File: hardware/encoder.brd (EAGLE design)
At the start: 26.2 x 31.4 mm, 13 parts

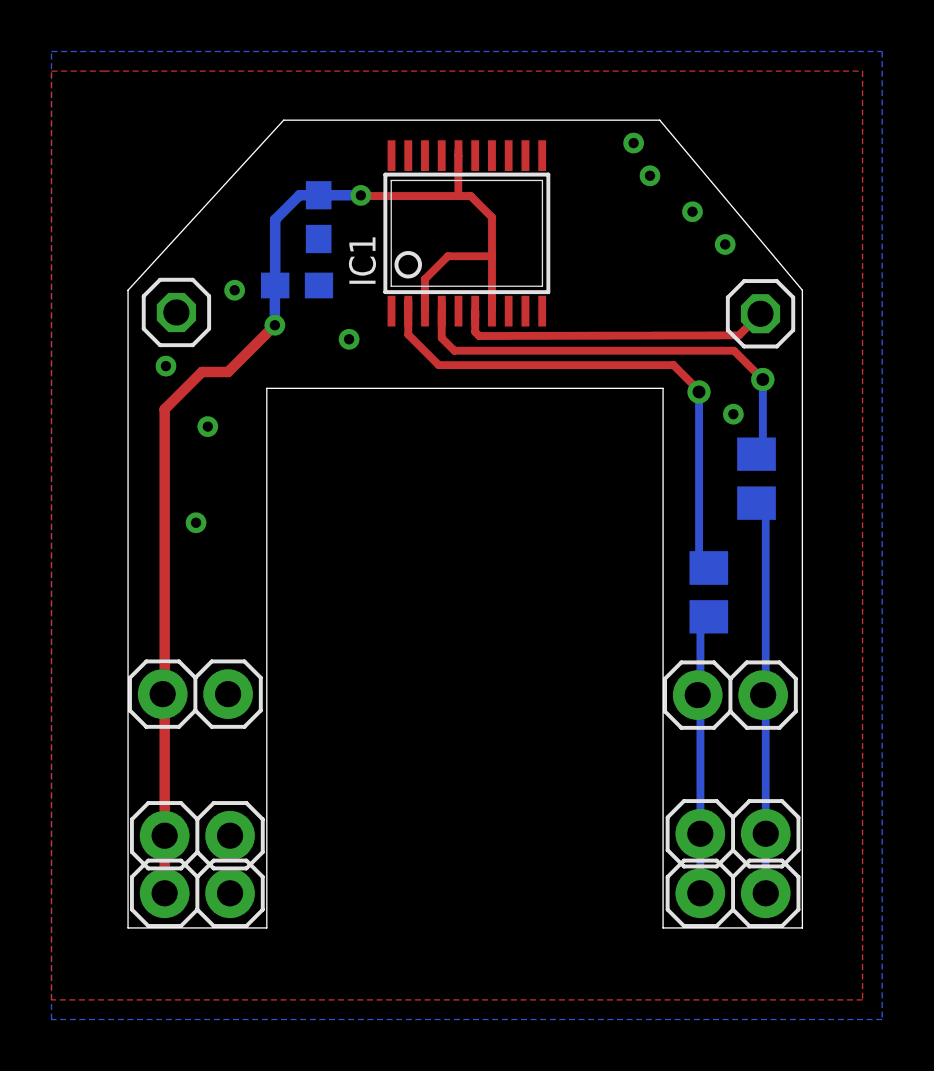
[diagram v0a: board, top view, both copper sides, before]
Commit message: new driver
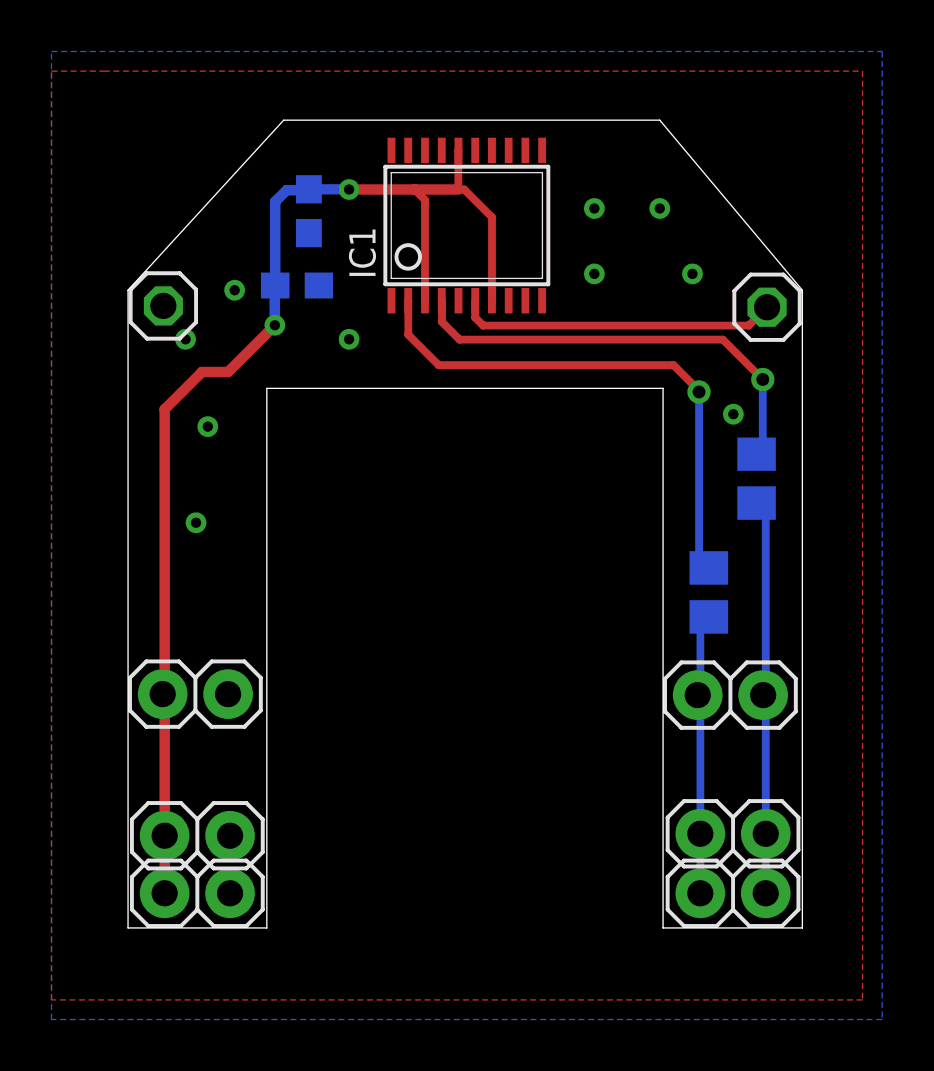
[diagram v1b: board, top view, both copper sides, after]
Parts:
- moved JP8 0.57 mm to (11.2, 24.2)
- moved C1 0.44 mm to (16.9, 27.8)
- moved JP3 0.36 mm to (34.6, 24.1)
- moved IC1 0.30 mm to (23.0, 27.3)

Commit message: poprawilem enkodery
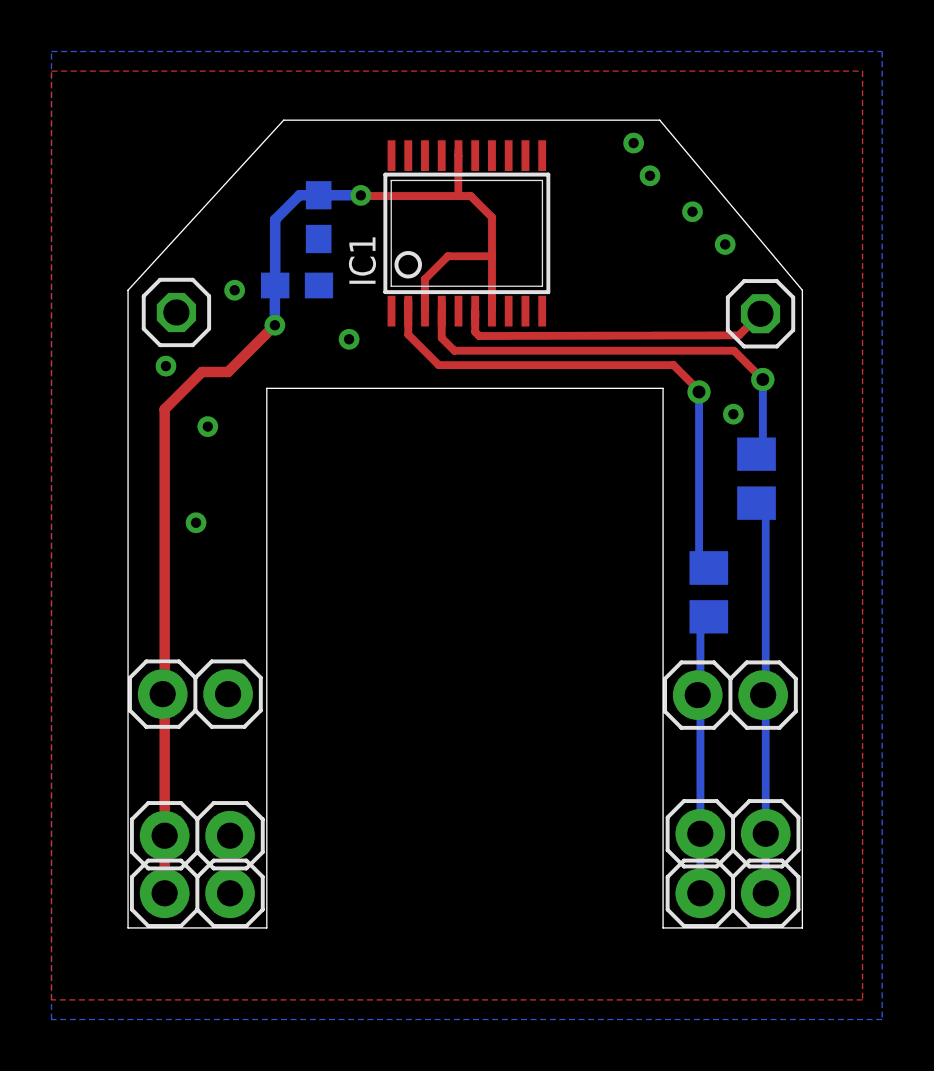
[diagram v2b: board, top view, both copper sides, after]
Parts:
- moved JP8 0.57 mm to (11.7, 23.9)
- moved C1 0.44 mm to (17.2, 27.6)
- moved JP3 0.36 mm to (34.4, 23.9)
- moved IC1 0.30 mm to (23.0, 27.0)
